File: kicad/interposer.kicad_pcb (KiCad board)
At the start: 2 copper layers, 18.3 x 39.7 mm, 22 parts, among them J1 Dial, J2 Stove, J3 Stove, Q1 2N7002, U1 XIAO-nRF52840-DIP, U2 MCP6042-E_SN, U3 TXU0101DBVR, U4 TMUX1119DBVR

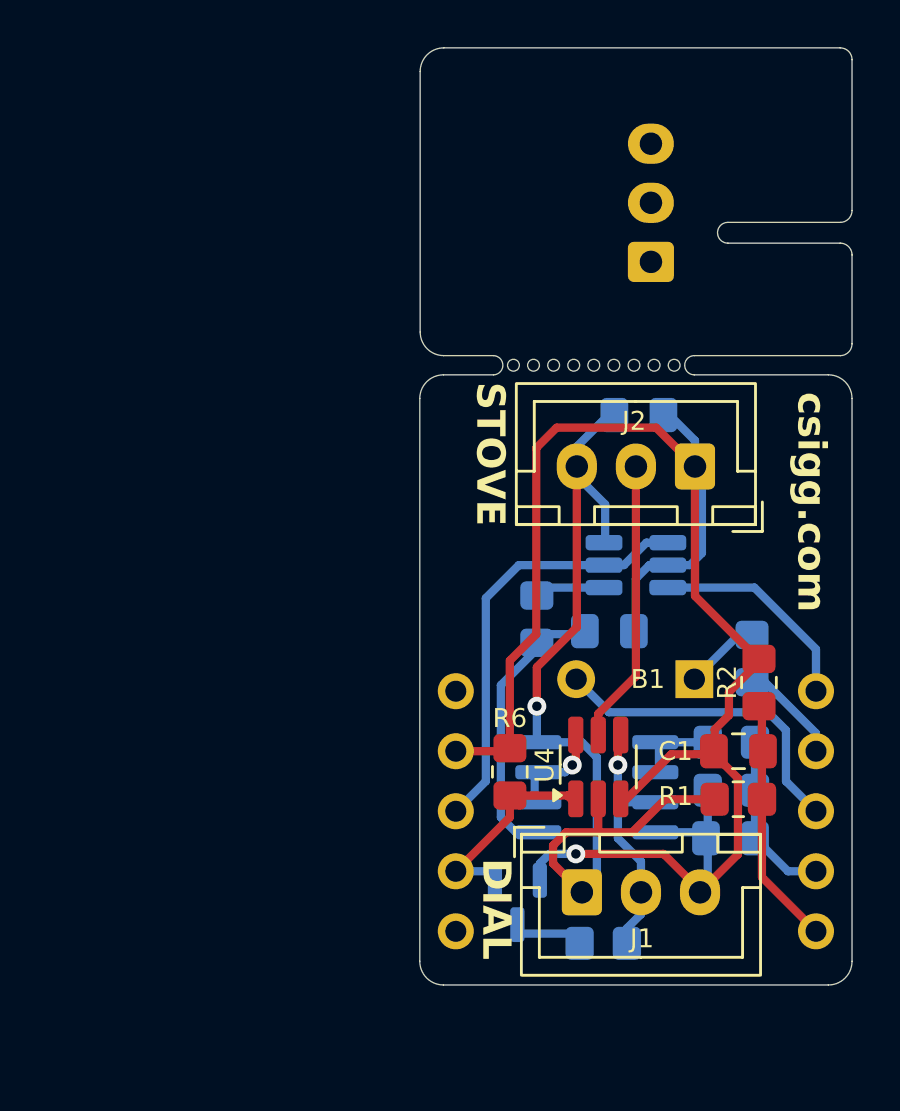
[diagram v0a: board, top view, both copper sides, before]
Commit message: Update KiCad
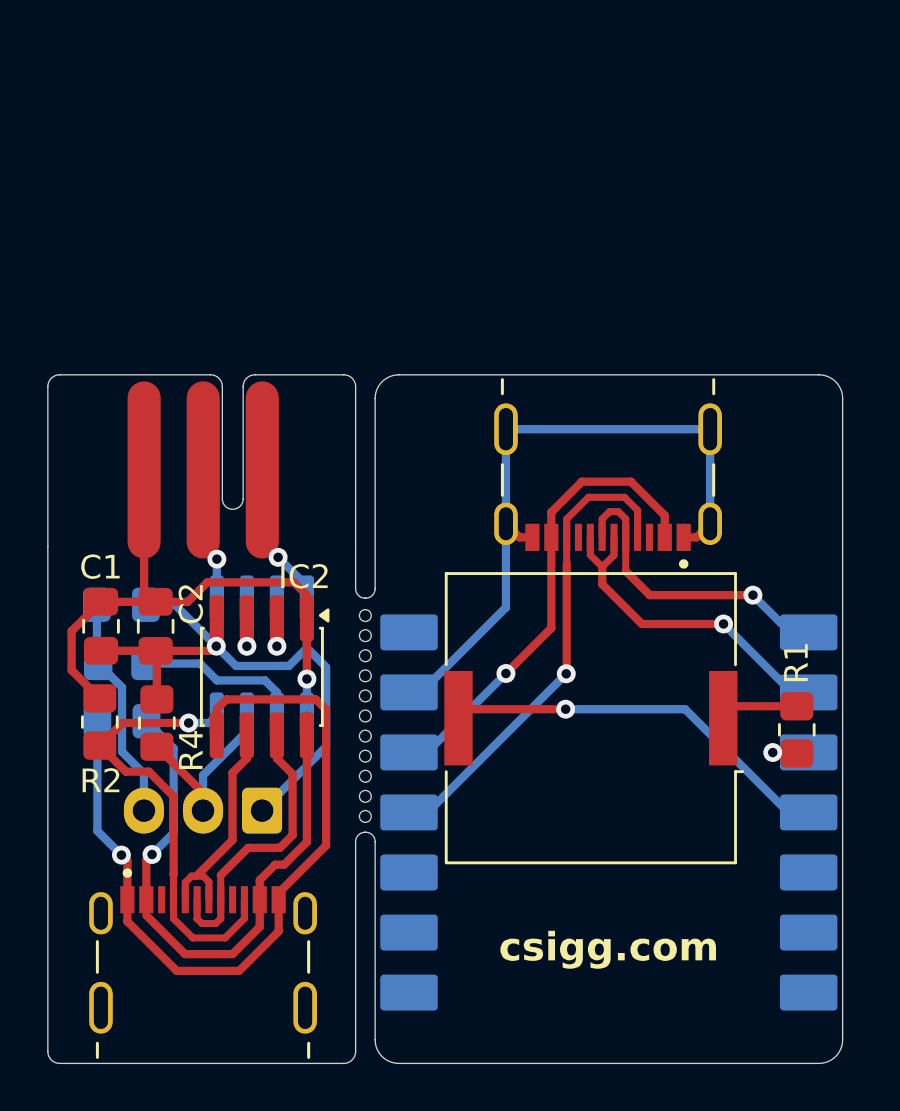
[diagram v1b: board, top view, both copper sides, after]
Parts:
- removed the J2 at (126.2, 73.2)
- removed Q1: 2N7002, Package_TO_SOT_SMD:SOT-23
- removed the R1 at (128.0, 87.2)
- removed R5: 33kΩ, Resistor_SMD:R_0805_2012Metric_Pad1.20x1.40mm_HandSolder
- removed R6: 100kΩ, Resistor_SMD:R_0805_2012Metric_Pad1.20x1.40mm_HandSolder
- removed R8: 1MΩ, Resistor_SMD:R_0805_2012Metric_Pad1.20x1.40mm_HandSolder
- removed the REF** at (121.9, 68.9)
- removed U2: MCP6042-E_SN, Package_SO:SOIC-8_3.9x4.9mm_P1.27mm
- removed U3: TXU0101DBVR, Package_TO_SOT_SMD:SOT-23-6_Handsoldering
- removed U4: TMUX1119DBVR, Package_TO_SOT_SMD:SOT-23-6_Handsoldering
- added IC1: PIC16F17114-I_SN, Package_SO:SOIC-8_3.9x4.9mm_P1.27mm, B.Cu at (107.9, 81.2)
- added IC2: ISO7021DR, Package_SO:SOIC-8_3.9x4.9mm_P1.27mm, F.Cu at (107.9, 82.1)
- added J1: PADS_STOVE_SIG, interposer:RAST 2.5 Pads, F.Cu at (105.4, 76.6)
- added J4: USB_XIAO, interposer:SAMESKY_UJ20-C-H-G-SMT-P16-TR, F.Cu at (122.5, 69.5)
- added REF**: BreakLine_11h_D0.5mm_P0.85mm, Panelization:BreakLine_11h_D0.5mm_P0.85mm, F.Cu at (112.2, 83.7)
- B1: footprint interposer:Buzzer_TDK_PS1240P02BT_D12.2mm_H6.5mm -> Buzzer_Beeper:Buzzer_Murata_PKLCS1212E
- C1: value 100nF -> 10µF
- C2: moved to F.Cu
- C3: value 1µF -> 10nF
- C4: value 1µF -> 100nF
- J2: renamed from J1; value Dial -> JST_DIAL; footprint Connector_JST:JST_XH_B3B-XH-A_1x03_P2.50mm_Vertical -> Connector_JST:JST_XH_S3B-XH-A_1x03_P2.50mm_Horizontal; moved to B.Cu
- J3: value Stove -> USB_PIC; footprint Connector_JST:JST_XH_S3B-XH-A_1x03_P2.50mm_Horizontal -> interposer:SAMESKY_UJ20-C-H-G-SMT-P16-TR; moved to F.Cu
- R1: renamed from R7; value 100Ω -> 220Ω; moved to F.Cu
- R2: value 51kΩ -> 10kΩ
- R3: value 27kΩ -> 220Ω
- R4: value 51kΩ -> 270kΩ; moved to F.Cu
- moved J3 38.6 mm to (105.4, 98.2), turned to 0 degrees
- moved R2 27.9 mm to (101.0, 84.0)
- moved C1 27.5 mm to (101.1, 79.9), turned to -90 degrees
- moved R3 26.0 mm to (101.9, 81.5)
- moved C2 25.9 mm to (103.4, 79.9), turned to -90 degrees
- moved C4 25.4 mm to (102.0, 83.9), turned to 180 degrees
- moved R4 24.5 mm to (103.4, 84.0), turned to 90 degrees
- moved C3 20.7 mm to (101.9, 79.0)
- moved J2 14.0 mm to (107.9, 87.7), turned to 180 degrees
- moved B1 4.68 mm to (121.8, 83.8)
- moved R1 3.56 mm to (130.5, 84.3)
- moved U1 2.74 mm to (122.6, 87.8)
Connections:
- C1 pad 1: /REF -> +5V
- C1 pad 2: GND -> GND_PIC
- C2 pad 1: /READ -> +5V
- C2 pad 2: GND -> GND_PIC
- C3 pad 1: /RC -> /DIAL_REF
- C3 pad 2: GND -> GND_PIC
- C4 pad 1: +5V -> VBUS_ISO
- C4 pad 2: GND -> GND_ISO
- J2 pad 1: +5V -> GND_PIC
- J2 pad 2: /DIAL -> /DIAL_SIG
- J2 pad 3: GND -> /DIAL_REF
- R2 pad 1: /REF -> /PROG_PIC
- R2 pad 2: GND -> +5V
- R3 pad 1: /IN -> /DIAL_REF
- R3 pad 2: /READ -> /DIAL_EXC
- R4 pad 1: /READ -> /DIAL_SIG
- R4 pad 2: GND -> GND_PIC
- U1 pad 1: /PWM_3V3 -> /RX_XIAO
- U1 pad 11: /SEL -> /PROG_XIAO
- U1 pad 13: GND -> GND_XIAO
- U1 pad 2: /+BUZZ -> /TX_XIAO
- U1 pad 3: /-BUZZ -> /+BUZZ
- U1 pad 4: /READ -> /-BUZZ
- U1 pad 5: /REF -> unconnected-(U1-P0.04_A4_D4_SDA-Pad5)
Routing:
- net GND: track 74.0 -> 0.00 mm, vias 1 -> 0
- net GND_ISO: track 0.00 -> 33.0 mm, vias 0 -> 1
- net GND_XIAO: track 0.00 -> 28.0 mm
- net GND_PIC: track 0.00 -> 27.6 mm, vias 0 -> 2
- net VBUS_ISO: track 0.00 -> 24.5 mm, vias 0 -> 1
- net /PROG_XIAO: track 0.00 -> 19.6 mm, vias 0 -> 1
- net /PROG_PIC: track 0.00 -> 19.1 mm, vias 0 -> 1
- net +5V: track 39.1 -> 24.8 mm
- net /TX_XIAO: track 0.00 -> 13.3 mm, vias 0 -> 1
- net /STOVE: track 12.7 -> 0.00 mm
- net /RX_XIAO: track 0.00 -> 12.3 mm, vias 0 -> 1
- net /TX_ISO: track 0.00 -> 12.0 mm
- net /DIAL: track 11.1 -> 0.00 mm, vias 1 -> 0
- net /RC: track 11.1 -> 0.00 mm
- net /REF: track 10.5 -> 0.00 mm
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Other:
- board size 18.3 x 39.7 mm -> 33.6 x 29.1 mm
- board text removed: "Conn_Internal"
- board text removed: "DIAL"
- board text removed: "STOVE"
